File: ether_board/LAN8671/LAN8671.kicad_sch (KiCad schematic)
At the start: 39 parts, among them IC1 LAN8670C2-E_LMX, J1 Screw_Terminal_01x02

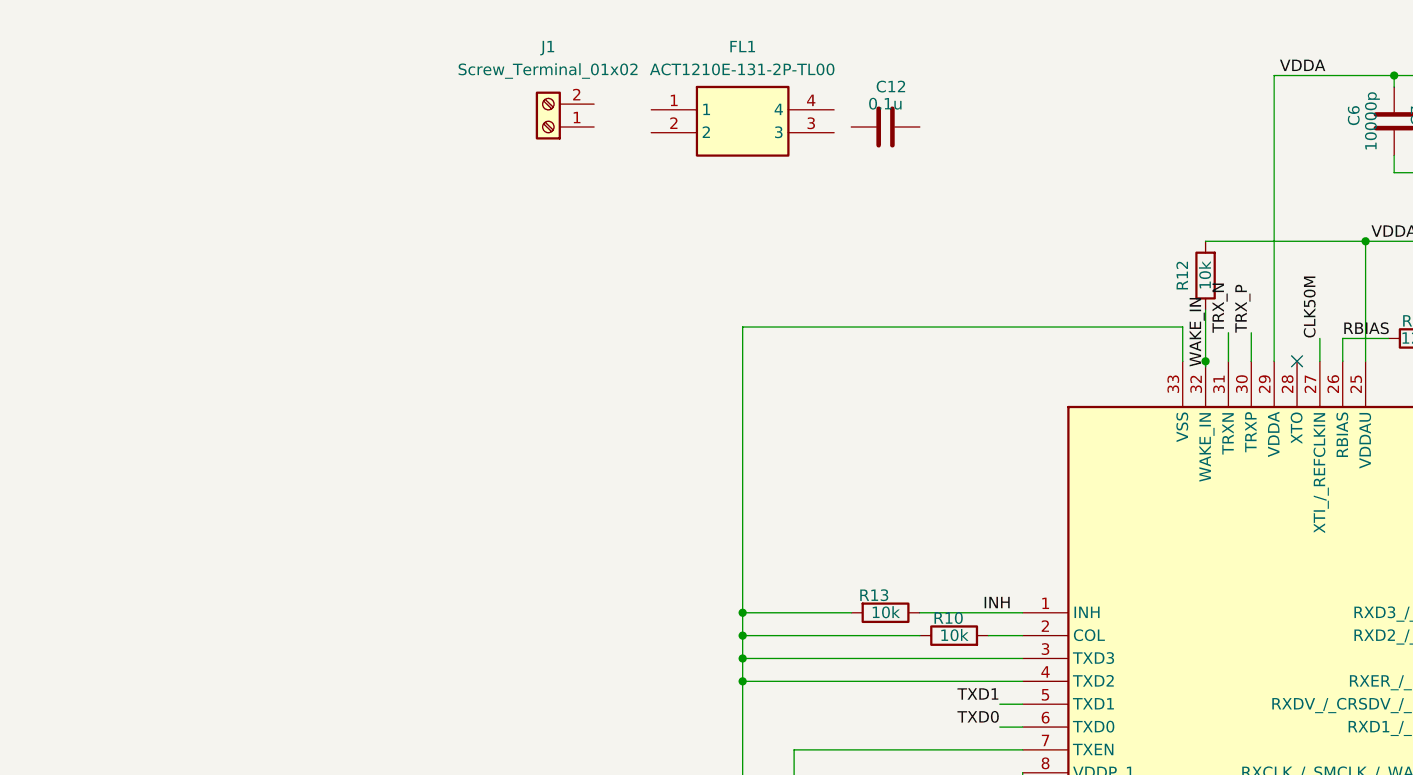
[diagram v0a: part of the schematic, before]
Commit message: edit shcematics
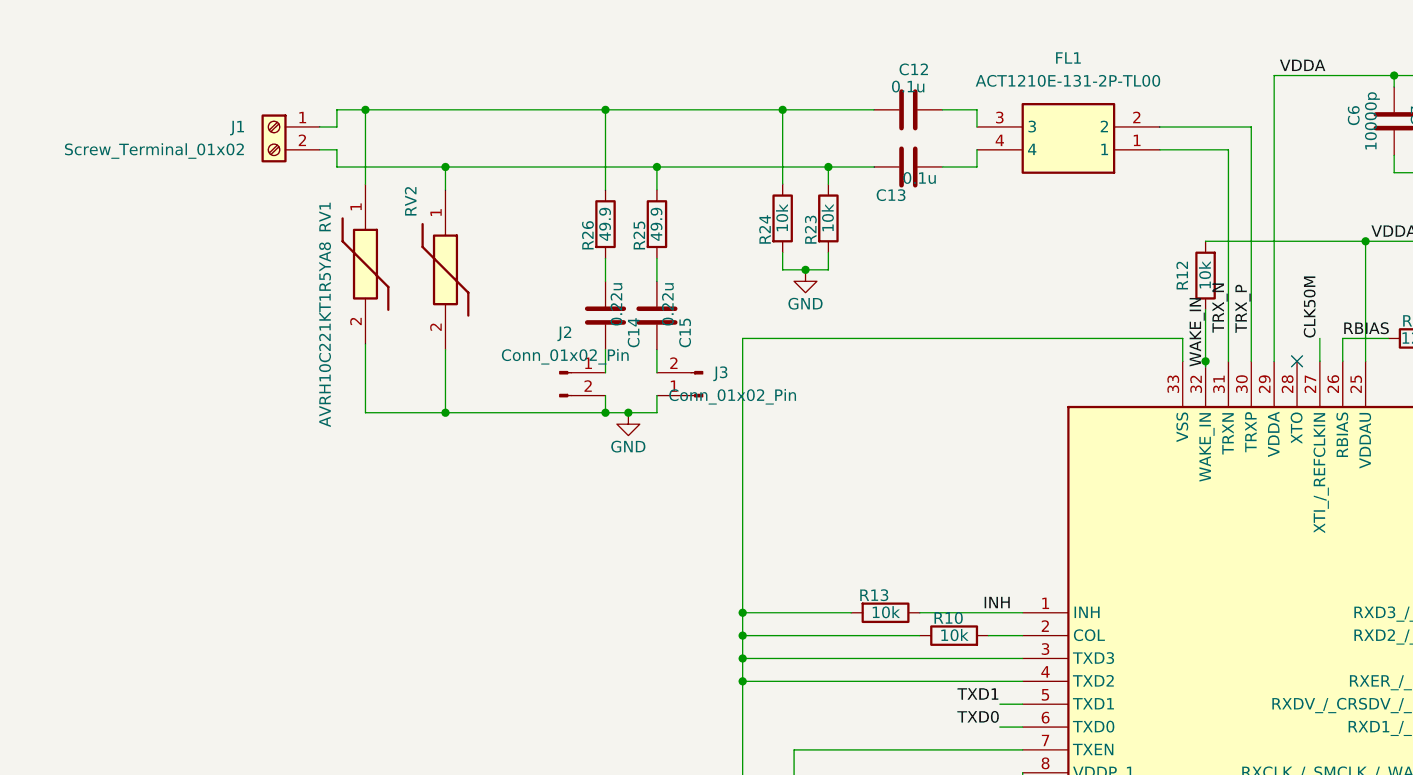
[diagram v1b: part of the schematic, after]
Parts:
- added C13: 0.1u, Capacitor_SMD:C_0603_1608Metric_Pad1.08x0.95mm_HandSolder, symbol Device:C
- added C14, C15: 0.22u, Capacitor_SMD:C_0603_1608Metric_Pad1.08x0.95mm_HandSolder, symbol Device:C
- added J2, J3: Conn_01x02_Pin, Connector_PinHeader_2.54mm:PinHeader_1x02_P2.54mm_Vertical, symbol Connector:Conn_01x02_Pin
- added R23, R24: 10k, Resistor_SMD:R_0603_1608Metric_Pad0.98x0.95mm_HandSolder, symbol Device:R
- added R25, R26: 49.9, Resistor_SMD:R_0603_1608Metric_Pad0.98x0.95mm_HandSolder, symbol Device:R
- added RV1, RV2: AVRH10C221KT1R5YA8, RESC1005X55N, symbol samacsys:AVRH10C221KT1R5YA8
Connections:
- net GND: now also J2.2 (Pin_2), J3.1 (Pin_1), R23.2, R24.2, RV1.2, RV2.2
- net TRX_N: now also FL1.1
- net TRX_P: now also FL1.2
- net at C12.1: now also J1.1 (Pin_1), R24.1, R26.1, RV1.1
- net at C12.2: now also FL1.3
- net at J1.2 (Pin_2): now also C13.1, R23.1, R25.1, RV2.1
- net at FL1.4: now also C13.2
- new net: C15.2, R25.2
- new net: C15.1, J3.2 (Pin_2)
- new net: C14.1, J2.1 (Pin_1)
- new net: C14.2, R26.2
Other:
- moved on the sheet: C12, FL1, J1
